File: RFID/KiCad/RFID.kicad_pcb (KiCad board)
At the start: 2 copper layers, 52.1 x 15.5 mm, 4 parts, among them J1 SPI IN, J3 SPI OUT

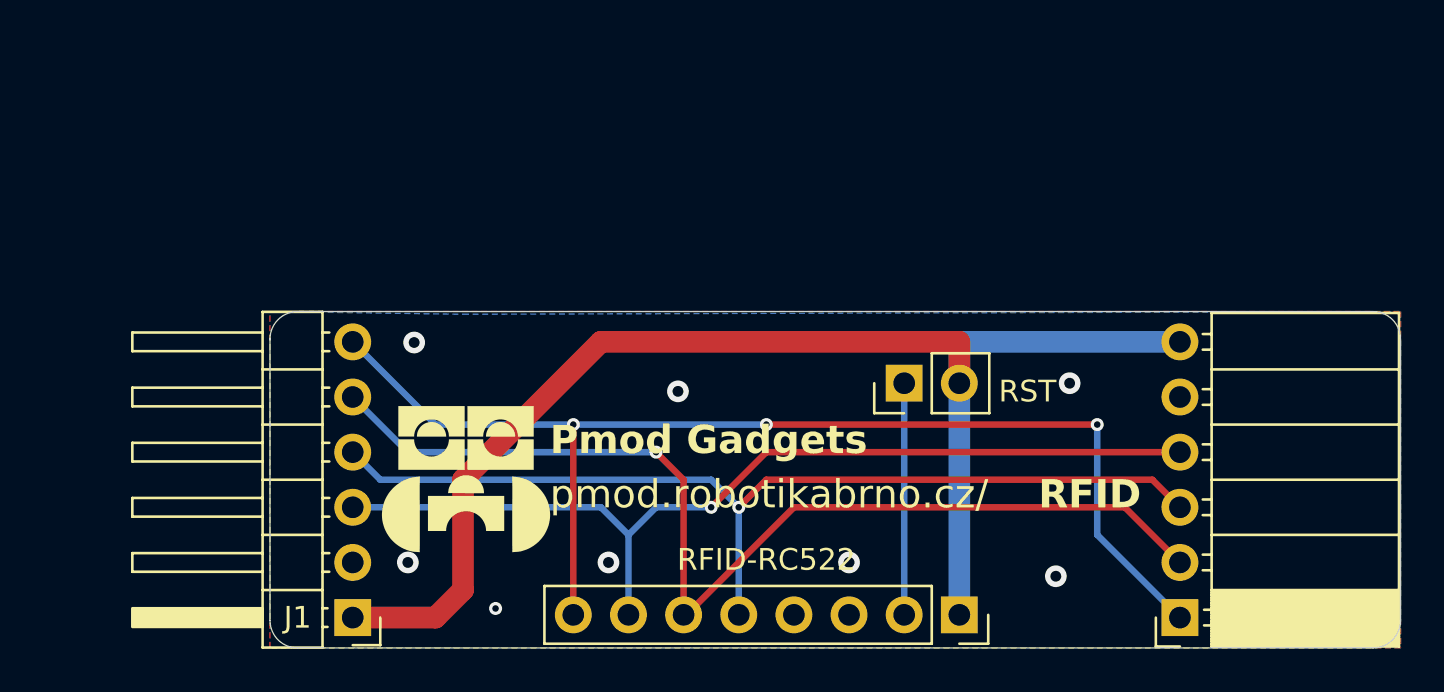
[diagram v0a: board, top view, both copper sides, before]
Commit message: Deployed d972a79 with MkDocs version: 1.6.0
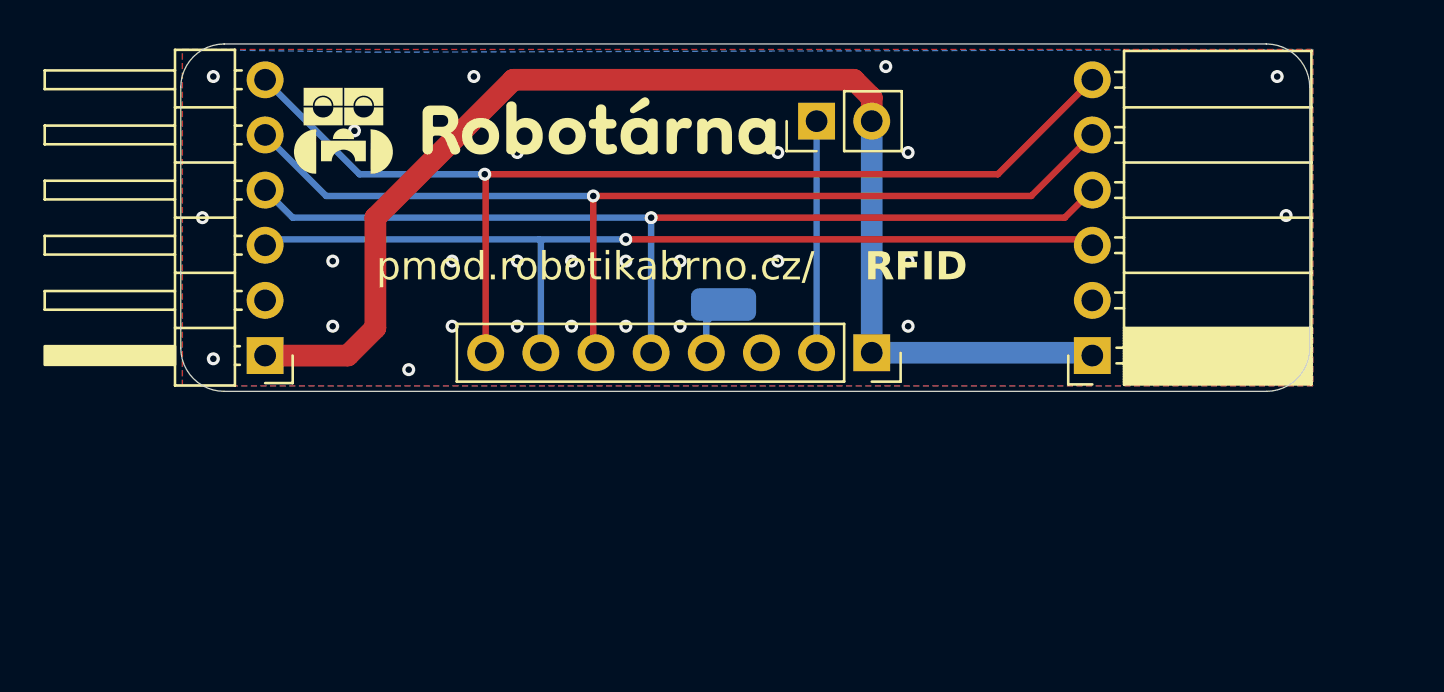
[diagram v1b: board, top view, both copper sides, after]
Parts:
- added TR1: 1KQ, Connector_Wire:SolderWirePad_1x01_SMD_1.5x3mm, B.Cu at (75.5, 44.0)
- moved J1 12.7 mm to (54.4, 46.4)
- moved J2 12.7 mm to (82.3, 46.2)
- moved J3 12.7 mm to (92.5, 46.4)
- moved J4 12.7 mm to (79.8, 35.6)
- renumbered RFID-RC522 to J2, RST to J4
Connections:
- J3 pad 1: SS -> +3.3V
- J3 pad 2: MOSI -> GND
- J3 pad 3: MISO -> SCK
- J3 pad 4: SCK -> MISO
- J3 pad 5: GND -> MOSI
- J3 pad 6: +3.3V -> SS
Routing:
- net SS: track 55.2 -> 50.1 mm, vias 3 -> 1
- net Net-(J2-Pin_4): track 0.00 -> 2.55 mm
- net +3.3V: track 60.3 -> 58.5 mm
- net MOSI: track 49.2 -> 47.7 mm
- net GND: vias 8 -> 28
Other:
- board size 52.1 x 15.5 mm -> 52 x 16 mm
- board text removed: "Pmod Gadgets"
